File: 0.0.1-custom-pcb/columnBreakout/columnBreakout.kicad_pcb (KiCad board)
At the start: 2 copper layers, 14 x 63 mm, 7 parts, among them J1 HC-FPC-0.5-12P-FH20, J2 HC-FPC-0.5-6P-FH20, J3 HC-FPC-0.5-6P-FH20, J4 HC-FPC-0.5-6P-FH20, J5 HC-FPC-0.5-6P-FH20, J6 HC-FPC-0.5-6P-FH20, J7 HC-FPC-0.5-6P-FH20

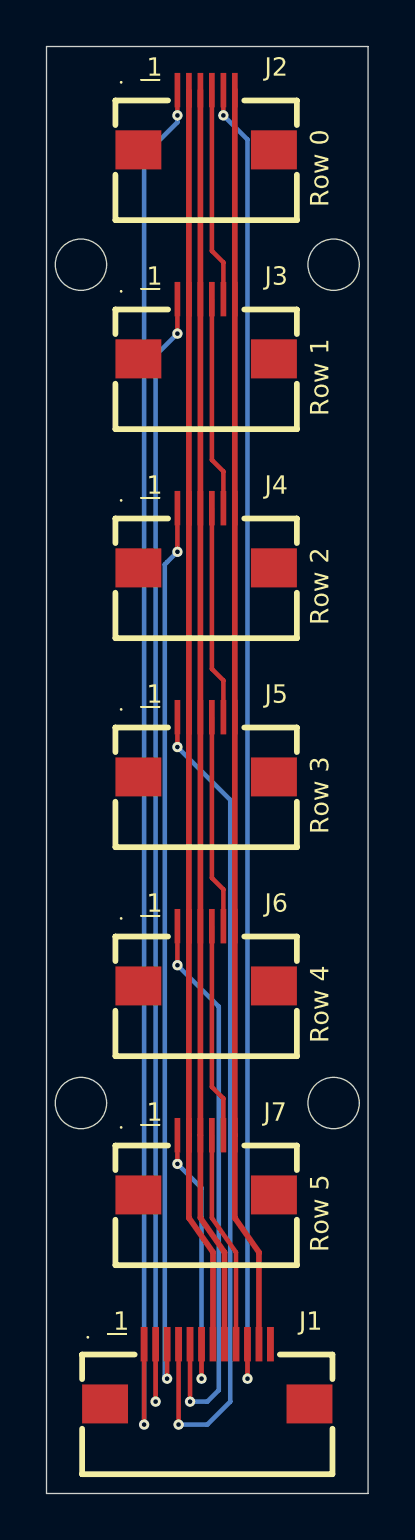
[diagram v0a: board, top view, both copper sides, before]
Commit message: final work before codex review
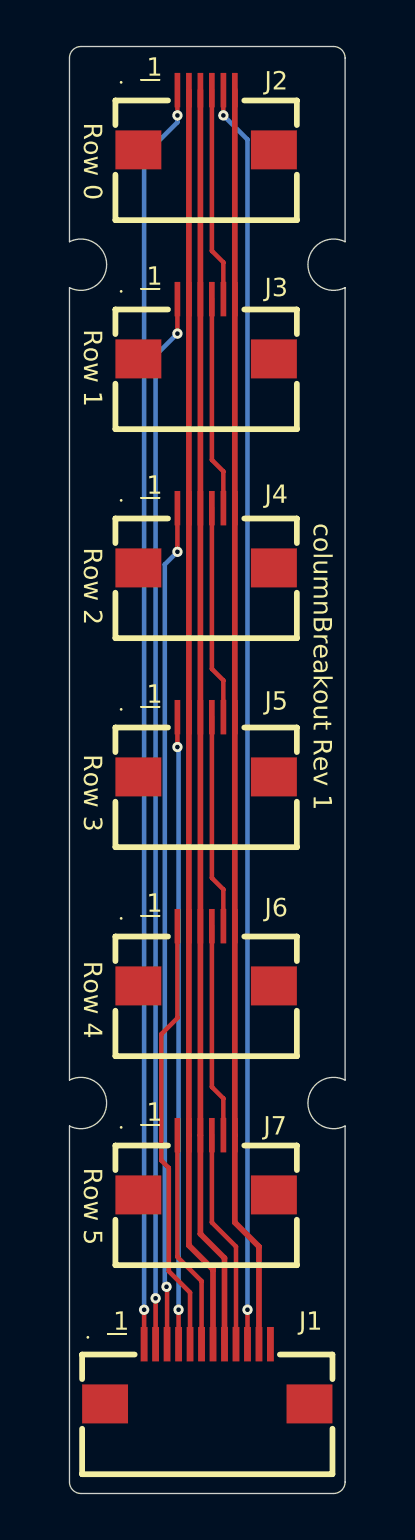
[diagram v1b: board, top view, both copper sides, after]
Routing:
- net /R3: track 36.9 -> 27.3 mm
- net /R0: track 62.2 -> 55.2 mm
- net /R4: track 24.9 -> 19.0 mm, vias 2 -> 0
- net /R1: track 50.9 -> 45.9 mm
- net /R2: track 39.7 -> 36.7 mm
- net /R5: track 12.5 -> 9.53 mm, vias 2 -> 0
- net /IN0: track 58.0 -> 55.0 mm
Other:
- board size 14 x 63 mm -> 12 x 63 mm
- board text added: "columnBreakout Rev 1"
